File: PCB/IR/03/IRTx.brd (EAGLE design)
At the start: 50 x 50 mm, 13 parts

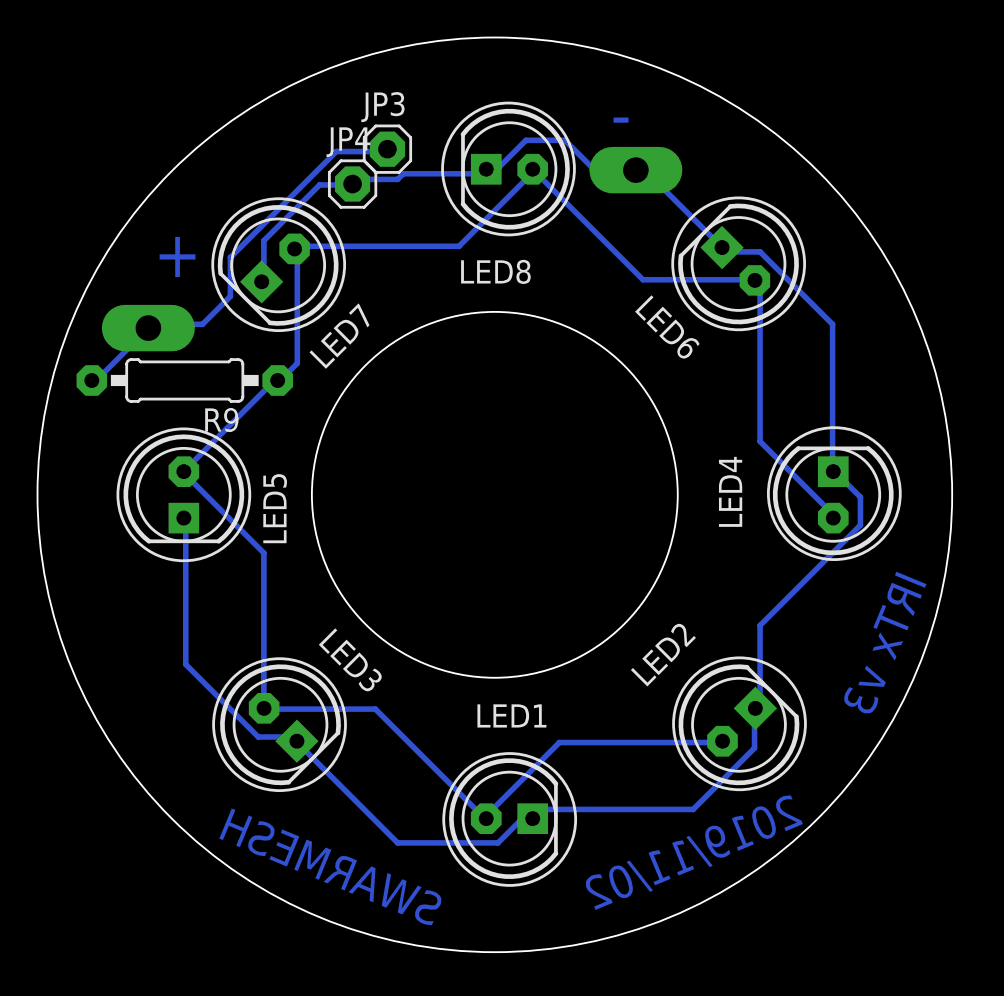
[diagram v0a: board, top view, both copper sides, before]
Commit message: modified IR-TX
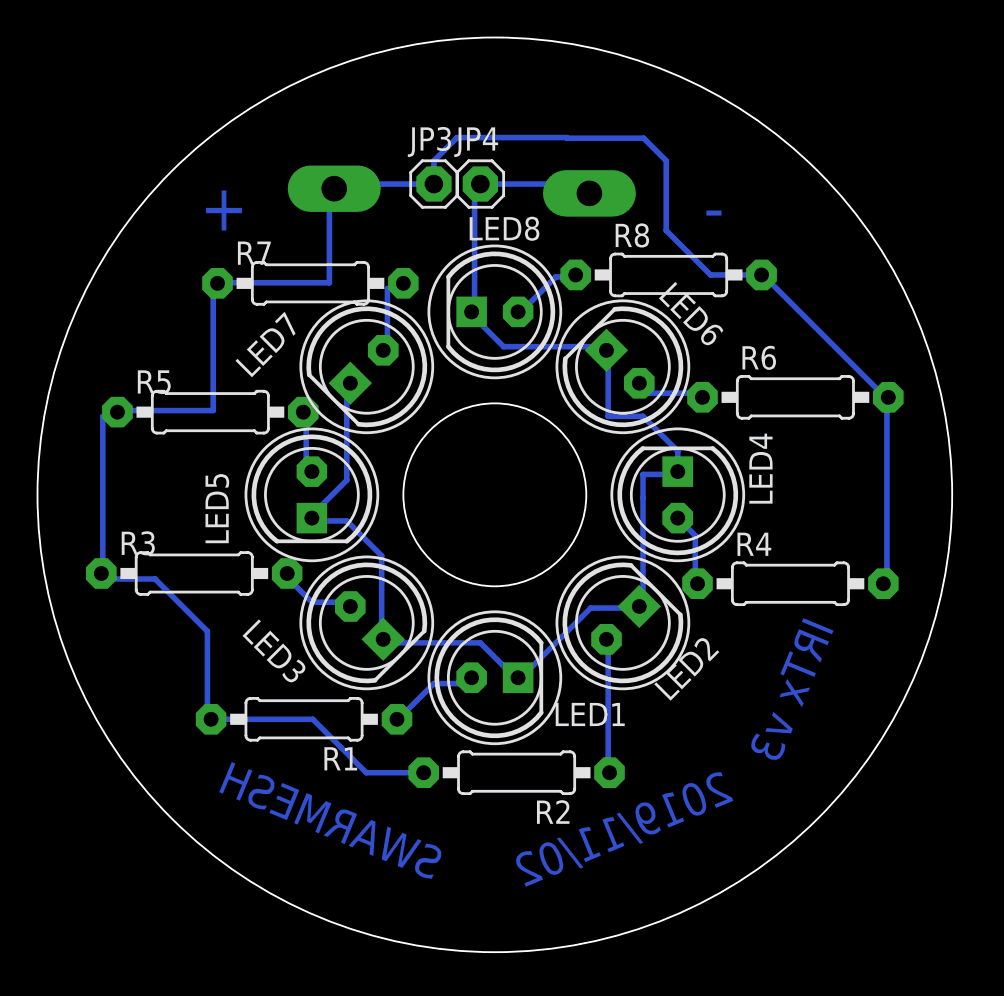
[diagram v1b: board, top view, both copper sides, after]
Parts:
- removed R9: 1k, adafruit:0207/10
- added R1, R2, R3, R4, R5, R6, R7, R8: 150, adafruit:0207/10
- moved JP1 12.7 mm to (21.2, 46.7)
- moved LED4 8.50 mm to (40.0, 30.0)
- moved LED6 8.46 mm to (37.0, 37.0)
- moved LED2 8.44 mm to (37.0, 23.0)
- moved LED8 7.84 mm to (30.0, 40.0)
- moved LED1 7.74 mm to (30.0, 20.0)
- moved LED7 7.36 mm to (23.0, 37.0)
- moved LED3 7.30 mm to (23.0, 23.0)
- moved LED5 7.00 mm to (20.0, 30.0)
- moved JP4 6.98 mm to (29.2, 47.0)
- moved JP3 3.18 mm to (26.7, 47.0)
- moved JP2 2.84 mm to (35.2, 46.5)
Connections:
- new net N$2: LED1.A, R1.1
- new net N$3: LED3.A, R3.1
- new net N$4: LED4.A, R4.1
- new net N$5: LED5.A, R5.1
- new net N$6: LED6.A, R6.1
- new net N$7: LED7.A, R7.1
- new net N$8: LED8.A, R8.1
- net N$1: now also R2.1; no longer LED1.A, LED3.A, LED4.A, LED5.A, LED6.A, LED7.A, LED8.A, R9.1
- net VCC: now also R1.2, R2.2, R3.2, R4.2, R5.2, R6.2, R7.2, R8.2; no longer R9.2
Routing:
- net N$1: track 103.4 -> 7.34 mm
- net VCC: track 22.7 -> 109.4 mm
- net GND: track 111.5 -> 74.6 mm
- net N$2: track 0.00 -> 5.08 mm
- net N$7: track 0.00 -> 4.49 mm
- net N$3: track 0.00 -> 4.31 mm
- net N$4: track 0.00 -> 4.01 mm
- net N$8: track 0.00 -> 3.98 mm
- net N$6: track 0.00 -> 3.85 mm
- net N$5: track 0.00 -> 3.49 mm
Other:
- outline, holes or cut-outs redrawn
